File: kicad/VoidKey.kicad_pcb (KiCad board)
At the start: 2 copper layers, 12 x 40 mm, 36 parts, among them J1 DEBUG, P1 Conn_USB_A_Plain, SW1 SW_Push, SW2 SW_Push, U1 RP2350_60QFN, U3 W25Q16JVZPIQ, U4 MCP1700T-3302E-TT, Y1 12MHz

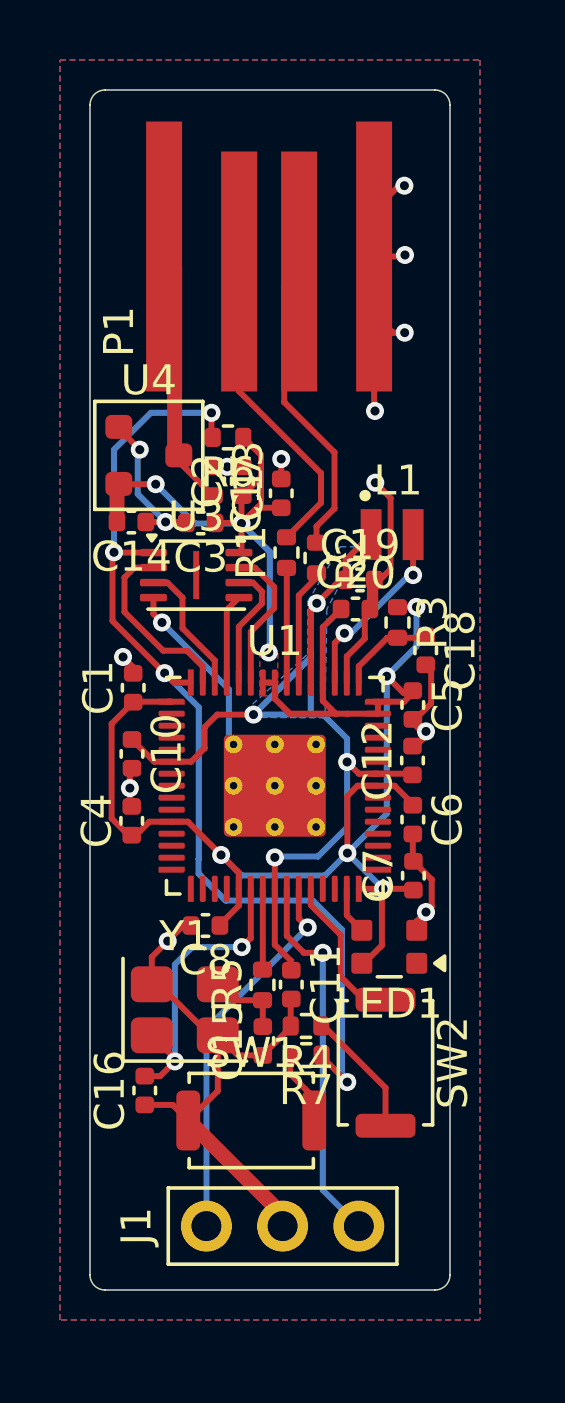
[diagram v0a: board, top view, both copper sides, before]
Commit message: fix: kicad sheet
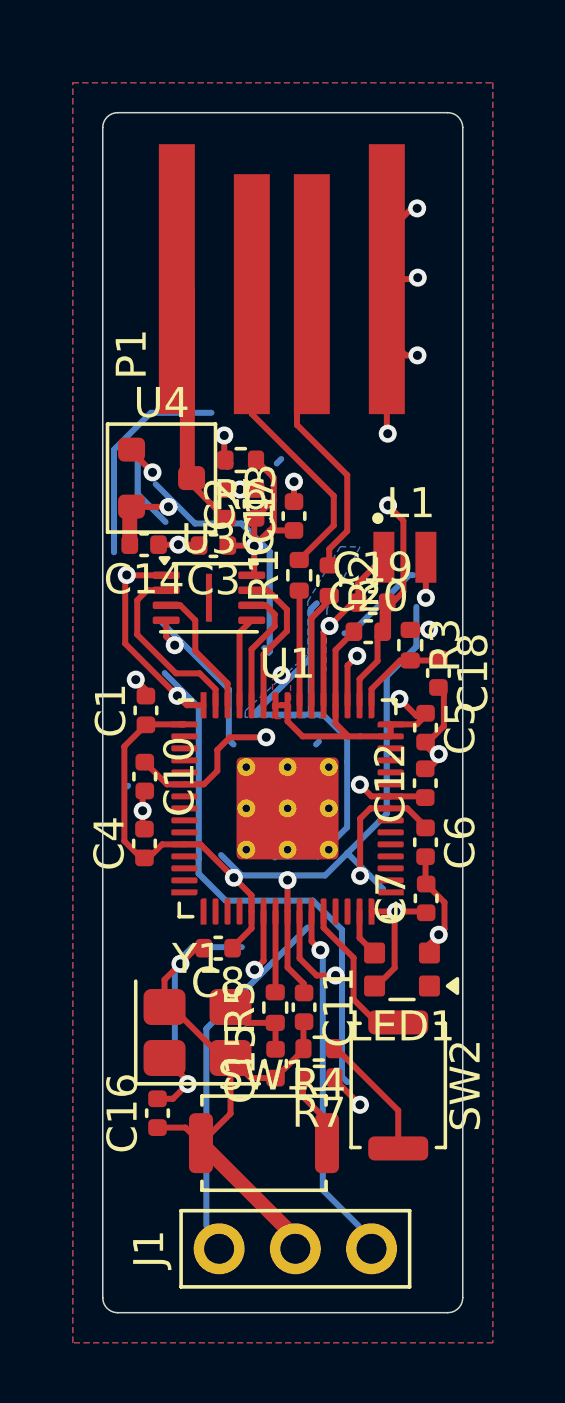
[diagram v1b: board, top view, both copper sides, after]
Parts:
- moved C19 0.87 mm to (23.4, 31.1)
- moved J1 0.87 mm to (18.3, 52.6)
- moved LED1 0.87 mm to (24.4, 43.3)
- moved R3 0.87 mm to (24.7, 32.5)
- moved R5 0.87 mm to (20.2, 44.6)
- moved C1 0.87 mm to (15.9, 34.7)
- moved C14 0.87 mm to (15.8, 29.2)
- moved C4 0.87 mm to (15.8, 39.1)
- moved C11 0.87 mm to (21.1, 44.6)
- moved C18 0.87 mm to (25.6, 33.4)
- moved C5 0.87 mm to (25.2, 35.3)
- moved C6 0.87 mm to (25.2, 39.1)
- moved C7 0.87 mm to (25.2, 40.9)
- moved R6 0.87 mm to (19.0, 26.3)
- moved SW2 0.87 mm to (24.3, 47.2)
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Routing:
- net GND: track 62.9 -> 84.5 mm, vias 15 -> 16
- net +1V1: track 33.9 -> 18.0 mm
- net /XIN: track 10.3 -> 4.56 mm
- net +3V3: vias 8 -> 7
